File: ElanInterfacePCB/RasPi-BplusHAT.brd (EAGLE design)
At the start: 65 x 56 mm, 34 parts, among them K1 PIN20X2, Q1 310mA/60V/1.6Ω, Q10 1.1A/60V/600mΩ, Q11 310mA/60V/1.6Ω, Q12 1.1A/60V/600mΩ, Q2 1.1A/60V/600mΩ, Q3 310mA/60V/1.6Ω, Q4 1.1A/60V/600mΩ, Q5 310mA/60V/1.6Ω, Q6 1.1A/60V/600mΩ, Q7 310mA/60V/1.6Ω, Q8 1.1A/60V/600mΩ, Q9 310mA/60V/1.6Ω, U2 MAX481CUA+

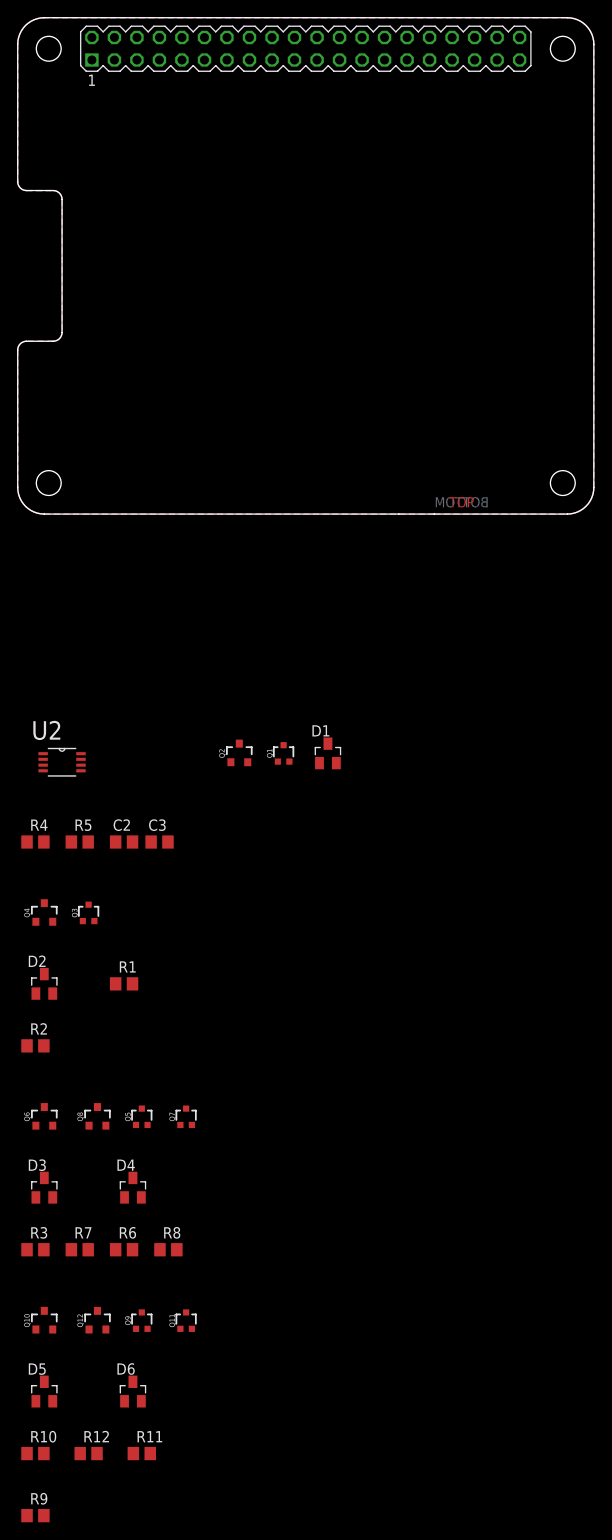
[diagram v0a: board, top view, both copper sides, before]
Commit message: Board Layout
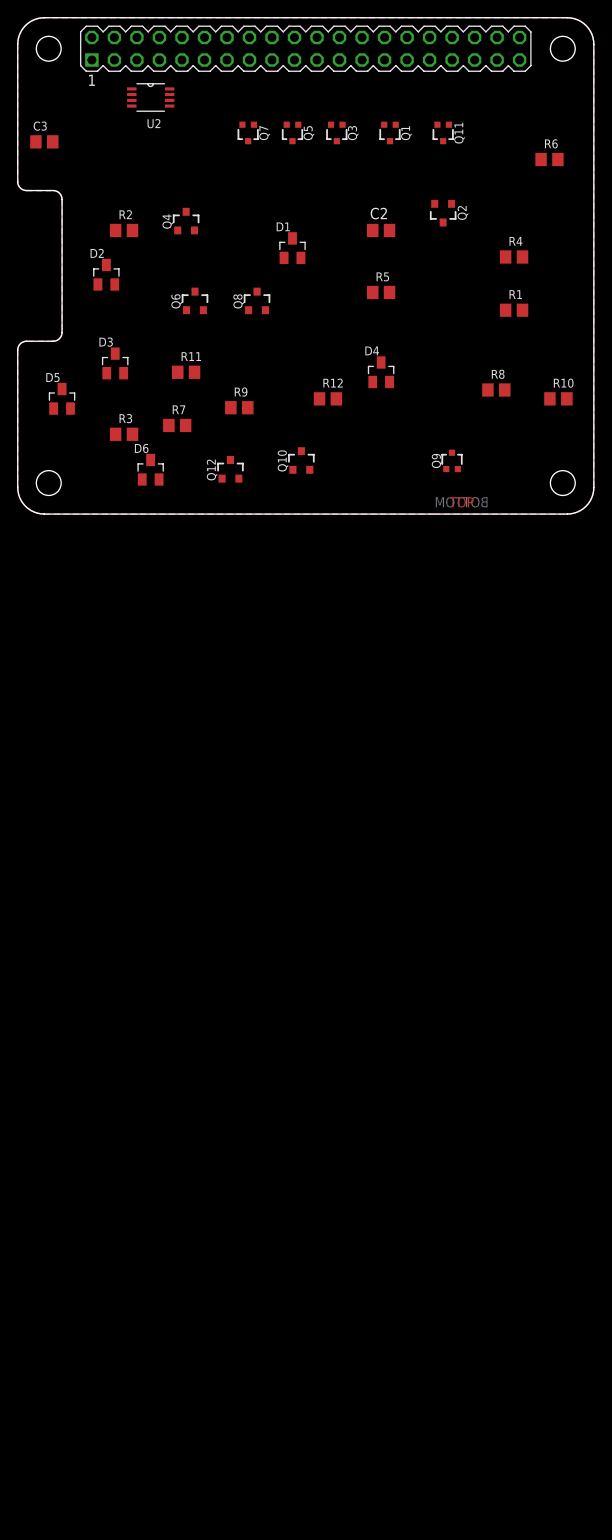
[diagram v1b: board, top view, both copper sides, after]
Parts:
- moved Q11 137.1 mm to (48.0, 43.0), turned to 180 degrees
- moved R10 132.8 mm to (61.0, 13.0)
- moved R6 132.0 mm to (60.0, 40.0)
- moved R9 127.1 mm to (25.0, 12.0)
- moved R11 122.1 mm to (19.0, 16.0)
- moved R12 122.0 mm to (35.0, 13.0)
- moved Q5 112.3 mm to (31.0, 43.0), turned to 180 degrees
- moved D5 112.0 mm to (5.00, 13.0)
- moved Q7 111.2 mm to (26.0, 43.0), turned to 180 degrees
- moved D6 104.0 mm to (15.0, 5.00)
- moved R8 103.8 mm to (54.0, 14.0)
- moved Q9 103.1 mm to (49.0, 6.00)
- moved Q10 101.2 mm to (32.0, 6.00)
- moved Q12 97.2 mm to (24.0, 5.00)
- moved D4 96.2 mm to (41.0, 16.0)
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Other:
- outline, holes or cut-outs redrawn
